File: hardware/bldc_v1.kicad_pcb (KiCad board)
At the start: 2 copper layers, 178.1 x 108.3 mm, 67 parts, among them J1 Conn_01x06, J2 1x2_ScrewTerminal_65A, J3 Screw_Terminal_01x05, J4 RJ45, J5 Screw_Terminal_01x03, M1 IPB017N10N5, M2 IPB017N10N5, M3 IPB017N10N5, M4 IPB017N10N5, M5 IPB017N10N5, M6 IPB017N10N5, M7 STM32F4-DISCOVERY, U1 AD8418, U2 AD8418

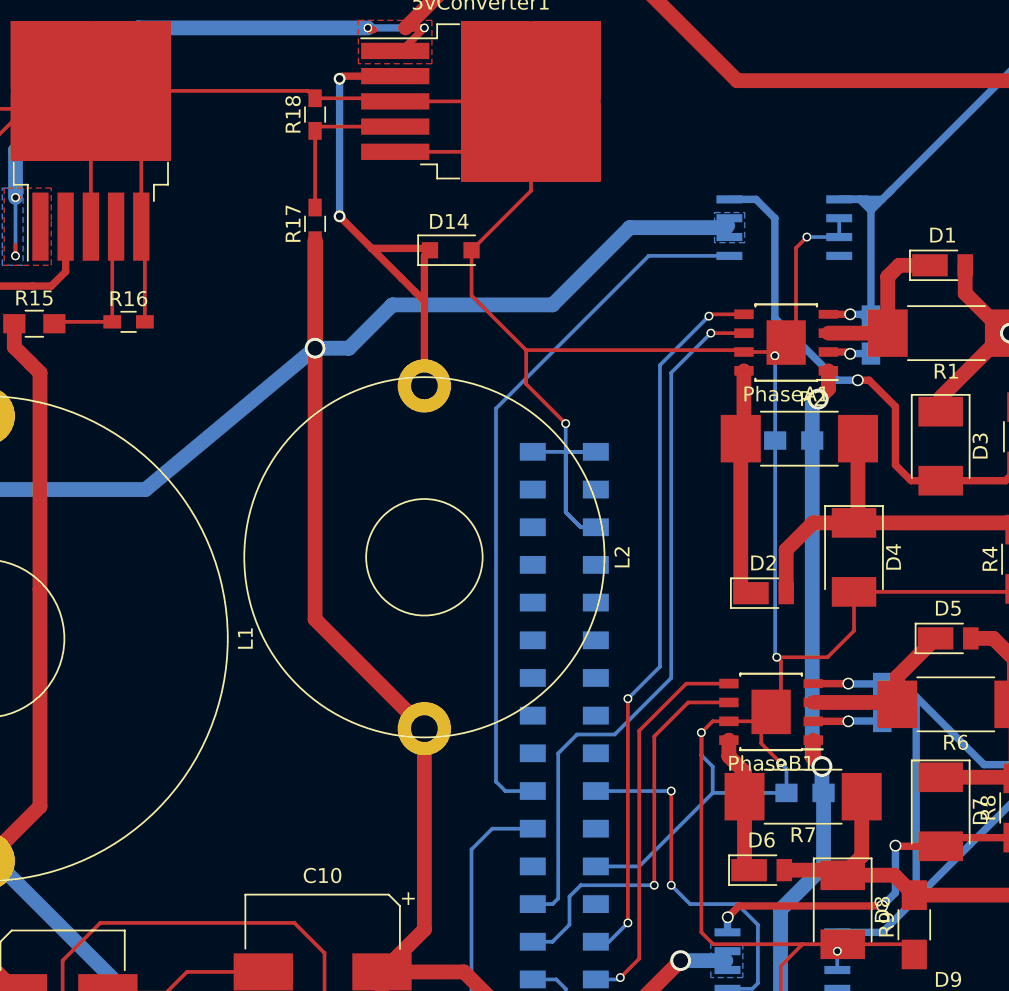
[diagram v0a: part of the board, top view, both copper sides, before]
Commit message: updated board layout
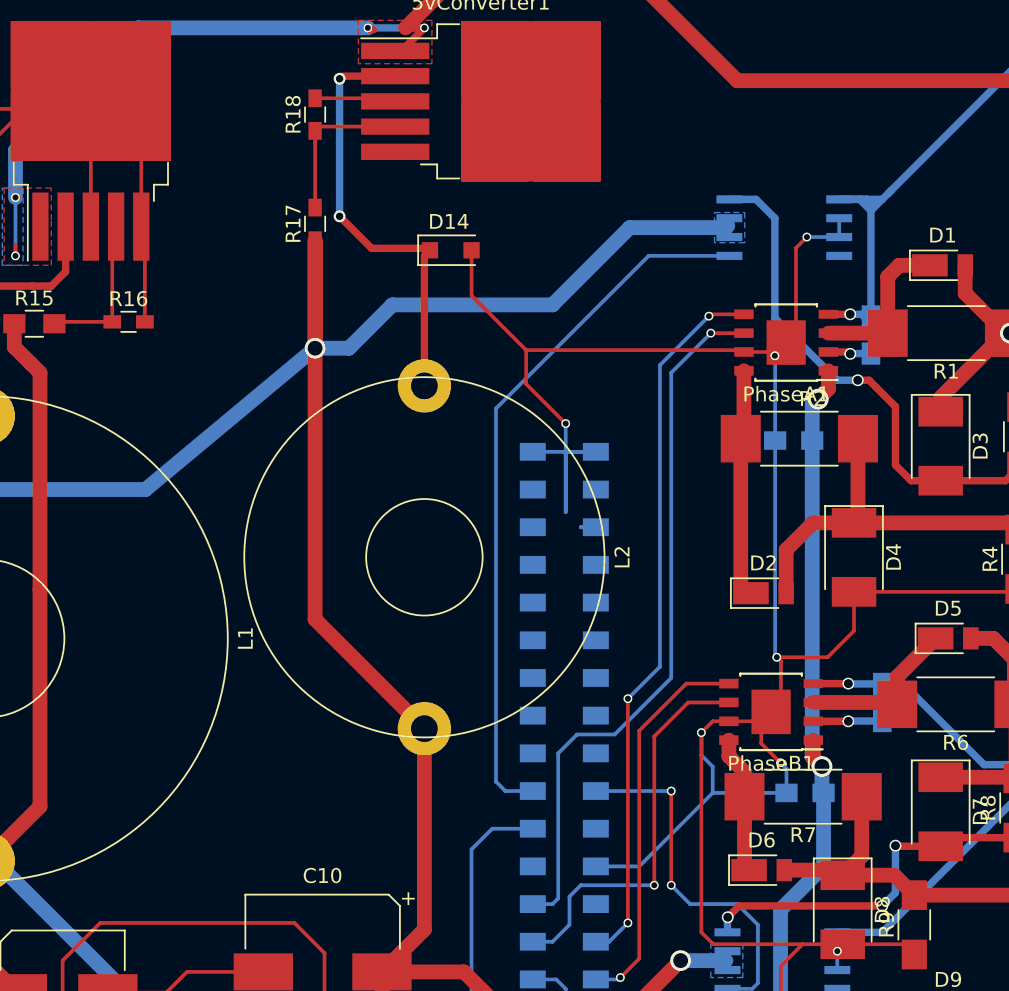
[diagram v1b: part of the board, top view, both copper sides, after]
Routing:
- net /GND: track 614.7 -> 569.9 mm
- net /GateDriver/PhaseB: track 170.1 -> 156.5 mm
- net Net-(5vConverter1-Pad2): track 34.5 -> 29.4 mm
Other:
- board text added: "Alex Simon BLDC Motor Controller 2/1/19 Rev 1"
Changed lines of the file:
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@@
     (area 72.336999 37.269 251.535001 149.325001)
     (thickness 1.6)
-    (drawings 8)
-    (tracks 901)
+    (drawings 9)
+    (tracks 889)
     (zones 0)
     (modules 67)
@@
   (layers
     (0 F.Cu signal)
-    (31 B.Cu signal)
+    (31 B.Cu signal hide)
     (32 B.Adhes user hide)
     (33 F.Adhes user hide)
@@
     (pad 1 np_thru_hole circle (at 0 0) (size 4.3 4.3) (drill 4.3) (layers *.Cu *.Mask))
   )
+  (gr_text "Alex Simon\nBLDC Motor Controller\n2/1/19\nRev 1" (at 235.204 116.332) (layer F.Mask)
+    (effects (font (size 1.5 1.5) (thickness 0.3)))
+  )
   (gr_line (start 157.861 139.192) (end 157.861 149.225) (angle 90) (layer Eco1.User) (width 0.2))
   (gr_line (start 251.46 37.846) (end 208.788 37.846) (angle 90) (layer Edge.Cuts) (width 0.15))
@@
   (segment (start 183.188 78.867) (end 192.338 78.867) (width 1) (layer F.Cu) (net 1))
   (segment (start 121.002 53.623) (end 120.59 53.623) (width 0.5) (layer F.Cu) (net 1))
-  (segment (start 118.999 66.929) (end 121.031 68.961) (width 0.5) (layer F.Cu) (net 2))
-  (segment (start 121.92 69.85) (end 122.555 70.485) (width 0.5) (layer F.Cu) (net 2))
-  (segment (start 121.031 68.961) (end 121.92 69.85) (width 0.5) (layer F.Cu) (net 2))
   (segment (start 120.59 55.323) (end 117.016 55.323) (width 0.5) (layer F.Cu) (net 2))
   (segment (start 118.999 66.929) (end 122.806 66.929) (width 0.5) (layer F.Cu) (net 2))
@@
   (segment (start 134.112 80.645) (end 132.08 80.645) (width 0.25) (layer B.Cu) (net 3))
   (segment (start 132.08 80.645) (end 132.08 84.709) (width 0.25) (layer B.Cu) (net 3))
-  (segment (start 132.08 84.709) (end 133.096 85.725) (width 0.25) (layer B.Cu) (net 3))
   (segment (start 133.096 85.725) (end 134.112 85.725) (width 0.25) (layer B.Cu) (net 3))
   (segment (start 83.312 141.605) (end 88.392 141.605) (width 0.25) (layer B.Cu) (net 3))
@@
   (segment (start 129.413 76.073) (end 129.413 73.787) (width 0.25) (layer F.Cu) (net 3))
   (segment (start 132.08 84.709) (end 132.08 80.772) (width 0.25) (layer B.Cu) (net 3))
-  (segment (start 133.096 85.725) (end 132.08 84.709) (width 0.25) (layer B.Cu) (net 3))
   (segment (start 134.112 85.725) (end 133.096 85.725) (width 0.25) (layer B.Cu) (net 3))
   (segment (start 129.862 80.645) (end 134.112 80.645) (width 0.25) (layer B.Cu) (net 3))
@@
   (segment (start 125.733 70.107) (end 129.413 73.787) (width 0.25) (layer F.Cu) (net 3))
   (segment (start 143.967 73.787) (end 144.094 73.914) (width 0.25) (layer F.Cu) (net 3))
-  (segment (start 129.74 57.023) (end 129.74 63.049) (width 0.25) (layer F.Cu) (net 3))
-  (segment (start 129.74 63.049) (end 125.733 67.056) (width 0.25) (layer F.Cu) (net 3))
   (segment (start 111.697 115.697) (end 106.553 115.697) (width 0.25) (layer F.Cu) (net 3))
   (segment (start 105.156 117.094) (end 101.221 117.094) (width 0.25) (layer F.Cu) (net 3))
@@
   (segment (start 83.312 56.007) (end 84.836 57.531) (width 0.25) (layer F.Cu) (net 3))
   (segment (start 98.86 57.531) (end 100.076 56.315) (width 0.25) (layer F.Cu) (net 3))
-  (segment (start 120.59 60.423) (end 126.34 60.423) (width 0.25) (layer F.Cu) (net 3))
   (segment (start 126.34 60.423) (end 129.74 57.023) (width 0.25) (layer F.Cu) (net 3))
   (segment (start 100.076 65.465) (end 100.076 56.315) (width 0.25) (layer F.Cu) (net 3))
   (segment (start 100.076 56.315) (end 103.476 59.715) (width 0.25) (layer F.Cu) (net 3))
   (segment (start 103.476 59.715) (end 103.476 65.465) (width 0.25) (layer F.Cu) (net 3))
-  (segment (start 100.076 56.315) (end 114.692 56.315) (width 0.25) (layer F.Cu) (net 3))
-  (segment (start 114.692 56.315) (end 115.189 56.812) (width 0.25) (layer F.Cu) (net 3))
-  (segment (start 120.59 57.023) (end 129.74 57.023) (width 0.25) (layer F.Cu) (net 3))
   (segment (start 115.189 56.812) (end 120.379 56.812) (width 0.25) (layer F.Cu) (net 3))
   (segment (start 120.379 56.812) (end 120.59 57.023) (width 0.25) (layer F.Cu) (net 3))
@@
   (segment (start 155.702 97.155) (end 154.833 96.286) (width 0.5) (layer B.Cu) (net 8))
   (segment (start 155.321 111.125) (end 155.702 110.744) (width 0.5) (layer B.Cu) (net 8))
-  (segment (start 155.702 110.744) (end 155.702 97.155) (width 0.5) (layer B.Cu) (net 8))
   (segment (start 148.768 96.266) (end 151.13 96.266) (width 0.5) (layer F.Cu) (net 8))
   (segment (start 151.15 96.286) (end 153.416 96.286) (width 0.5) (layer B.Cu) (net 8))
@@
   )
   (zone (net 3) (net_name /GND) (layer F.Cu) (hatch edge 0.508)
-    (connect_pads (clearance 0.35))
+    (connect_pads yes (clearance 0.35))
     (min_thickness 0.35)
     (fill yes (arc_segments 16) (thermal_gap 0.65) (thermal_bridge_width 0.4))
